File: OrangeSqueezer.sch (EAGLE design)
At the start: 31 parts, among them IC1 LM4558N, Q1 2N5457, Q2 2N5457

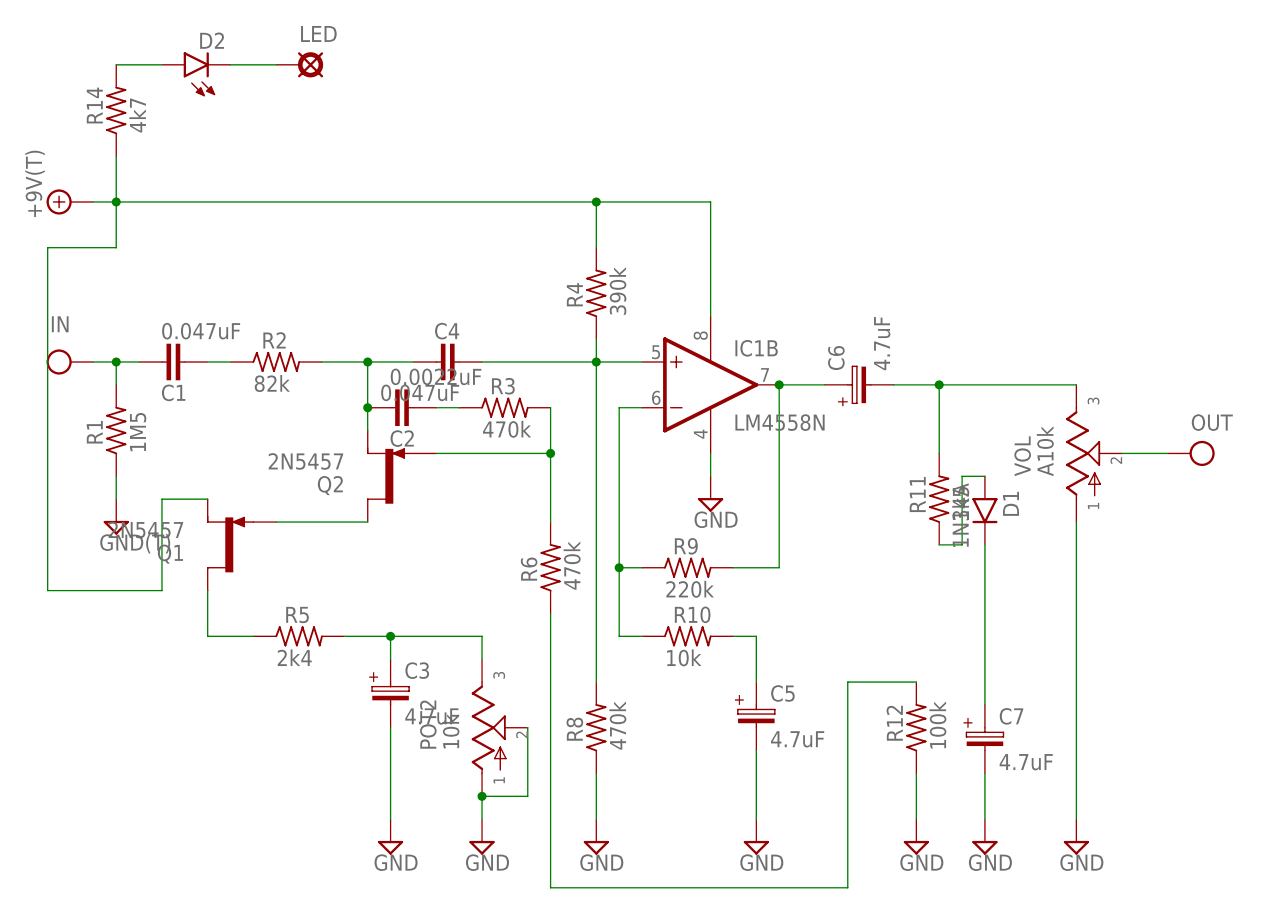
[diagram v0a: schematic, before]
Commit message: First commit for The Thing tremolo
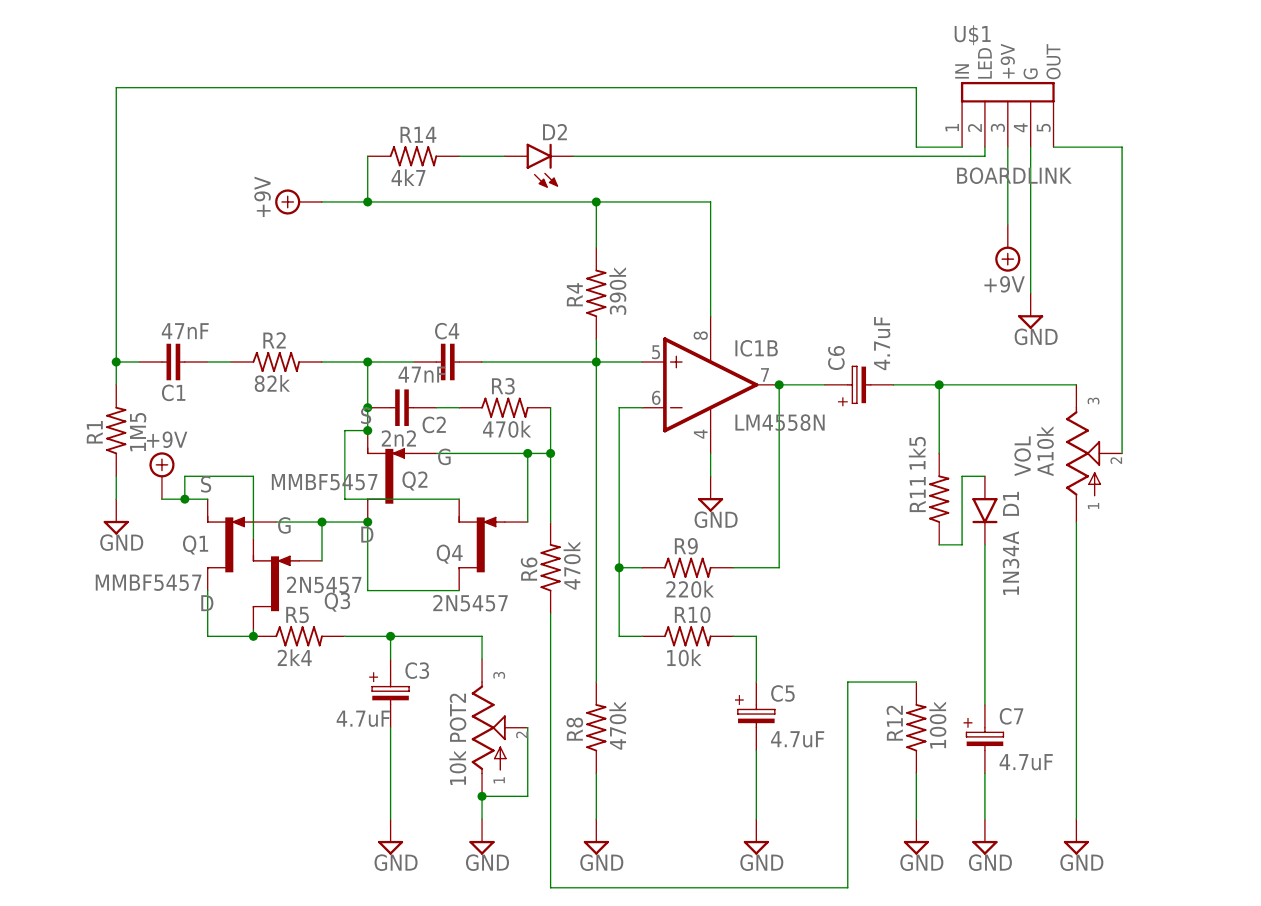
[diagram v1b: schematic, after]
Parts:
- removed +9V: +9V(T), mb_supply:+9V(T)
- removed G: GND(T), mb_supply:GND(T)
- removed IN: IN(T), mb_supply:IN(T)
- removed LED: LED, mb_supply:PAD
- removed OUT: OUT(T), mb_supply:OUT(T)
- added Q3, Q4: 2N5457, xc_library:2N5457
- added U$1: BOARDLINK, xc_library:BOARDLINK
- C1, C4: value 0.047uF -> 47nF
- C2: value 0.0022uF -> 2n2
- Q1, Q2: value 2N5457 -> MMBF5457; device mb_trans:2N5457 -> xc_library:MMBF5457
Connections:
- removed net IN: C1.2, IN.IN, R1.2
- removed net OUT: OUT.OUT, VOL.2
- new net N$10: U$1.OUT, VOL.2
- new net N$20: C1.2, R1.2, U$1.IN
- net +9V: now also Q3.S, U$1.+9V; no longer +9V.+9V
- net GND: now also U$1.G; no longer G.GND
- net N$16: now also U$1.LED; no longer LED.PAD
- net N$2: now also Q3.D
- net N$3: now also Q3.G, Q4.D
- net N$5: now also Q4.S
- net N$7: now also Q4.G
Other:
- moved on the sheet: D2, R14
